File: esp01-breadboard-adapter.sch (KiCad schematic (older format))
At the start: 4 parts, among them P1 CONN_02X04, P2 CONN_01X04, P3 CONN_01X04

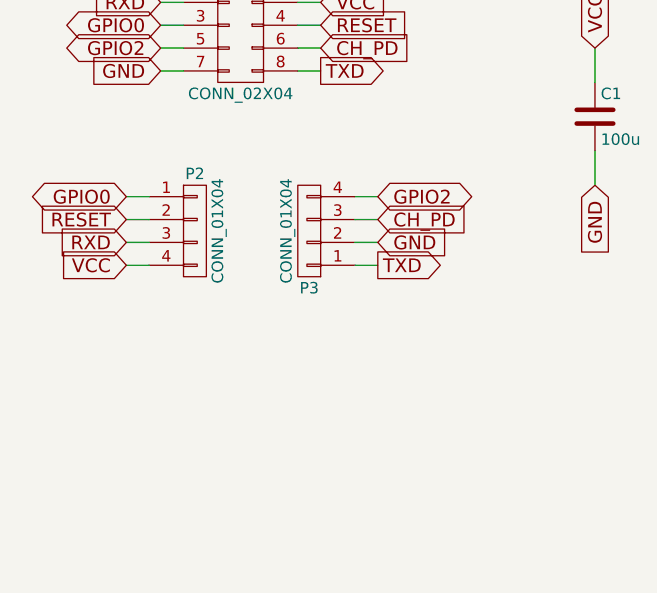
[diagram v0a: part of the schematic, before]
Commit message: edited schematic
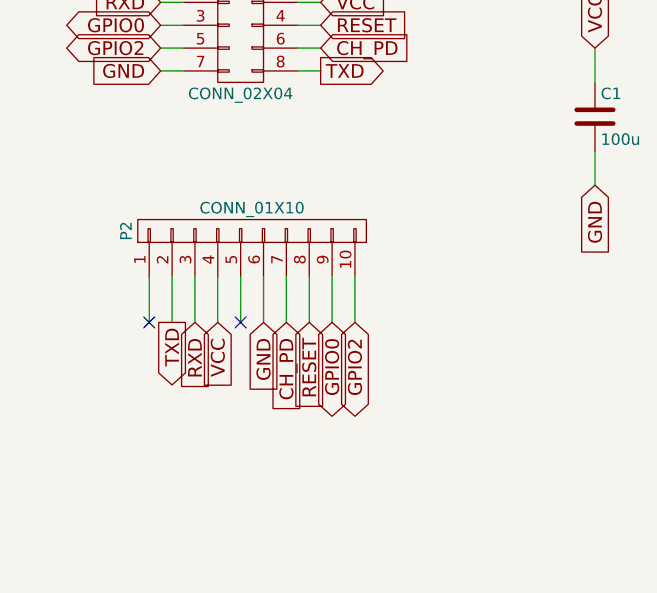
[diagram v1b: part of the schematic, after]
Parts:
- removed P2, P3: CONN_01X04, Pin_Headers:Pin_Header_Straight_1x04, symbol CONN_01X04
- added P2: CONN_01X10, Pin_Headers:Pin_Header_Straight_1x10, symbol CONN_01X10
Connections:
- net CH_PD: now also P2.7 (P7)
- net GND: now also P2.6 (P6)
- net GPIO0: now also P2.9 (P9)
- net GPIO2: now also P2.10 (P10)
- net RESET: now also P2.8 (P8)
- net RXD: now also P2.3 (P3)
- net TXD: now also P2.2 (P2)
- net VCC: now also P2.4 (P4)
- no-connect marks 0 -> 2
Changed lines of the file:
@@
 Francesco Urbani\n
 $Comp
-L CONN_01X04 P3
-U 1 1 585F9D0E
-P 5950 4150
-F 0 "P3" H 5950 4400 50  0000 C CNN
-F 1 "CONN_01X04" V 6050 4150 50  0000 C CNN
-F 2 "Pin_Headers:Pin_Header_Straight_1x04" H 5950 4150 50  0001 C CNN
-F 3 "" H 5950 4150 50  0000 C CNN
-	1    5950 4150
-	-1   0    0    1
+L CONN_01X10 P2
+U 1 1 5862AFF5
+P 5700 4150
+F 0 "P2" H 5700 4700 50  0000 C CNN
+F 1 "CONN_01X10" V 5800 4150 50  0000 C CNN
+F 2 "Pin_Headers:Pin_Header_Straight_1x10" H 5700 4150 50  0001 C CNN
+F 3 "" H 5700 4150 50  0000 C CNN
+	1    5700 4150
+	0    -1   -1   0
 $EndComp
-$Comp
-L CONN_01X04 P2
-U 1 1 585F9D14
-P 5450 4150
-F 0 "P2" H 5450 4400 50  0000 C CNN
-F 1 "CONN_01X04" V 5550 4150 50  0000 C CNN
-F 2 "Pin_Headers:Pin_Header_Straight_1x04" H 5450 4150 50  0001 C CNN
-F 3 "" H 5450 4150 50  0000 C CNN
-	1    5450 4150
-	1    0    0    -1
-$EndComp
+Text GLabel 5350 4550 3    60   Output ~ 0
+TXD
+Text GLabel 5450 4550 3    60   Input ~ 0
+RXD
+Text GLabel 5550 4550 3    60   Input ~ 0
+VCC
+Text GLabel 5750 4550 3    60   Input ~ 0
+GND
+Text GLabel 5850 4550 3    60   Input ~ 0
+CH_PD
+Text GLabel 5950 4550 3    60   Input ~ 0
+RESET
+Text GLabel 6050 4550 3    60   BiDi ~ 0
+GPIO0
+Text GLabel 6150 4550 3    60   BiDi ~ 0
+GPIO2
 Wire Wire Line
-	6150 4000 6250 4000
+	5350 4350 5350 4550
 Wire Wire Line
-	6150 4100 6250 4100
+	5450 4550 5450 4350
 Wire Wire Line
-	6150 4200 6250 4200
+	5550 4350 5550 4550
 Wire Wire Line
-	6150 4300 6250 4300
-Text GLabel 6250 4000 2    60   BiDi ~ 0
-GPIO2
-Text GLabel 6250 4100 2    60   Input ~ 0
-CH_PD
-Text GLabel 6250 4200 2    60   Input ~ 0
-GND
-Text GLabel 6250 4300 2    60   Output ~ 0
-TXD
+	5750 4550 5750 4350
 Wire Wire Line
-	5250 4300 5150 4300
+	5850 4350 5850 4550
 Wire Wire Line
-	5250 4200 5150 4200
+	5950 4550 5950 4350
 Wire Wire Line
-	5250 4100 5150 4100
+	6050 4350 6050 4550
 Wire Wire Line
-	5250 4000 5150 4000
-Text GLabel 5150 4000 0    60   BiDi ~ 0
-GPIO0
-Text GLabel 5150 4100 0    60   Input ~ 0
-RESET
-Text GLabel 5150 4200 0    60   Input ~ 0
-RXD
-Text GLabel 5150 4300 0    60   Input ~ 0
-VCC
+	6150 4550 6150 4350
+Wire Wire Line
+	5650 4350 5650 4550
+Wire Wire Line
+	5250 4550 5250 4350
+NoConn ~ 5650 4550
+NoConn ~ 5250 4550
 $EndSCHEMATC
